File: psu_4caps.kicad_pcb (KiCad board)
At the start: 2 copper layers, 112.5 x 72.5 mm, 38 parts, among them J1 AC1, J10 GND, J11 V-, J12 V-, J2 GND2, J3 GND3, J4 AC4, J5 LED, J6 LED, J7 V+, J8 V+, J9 GND

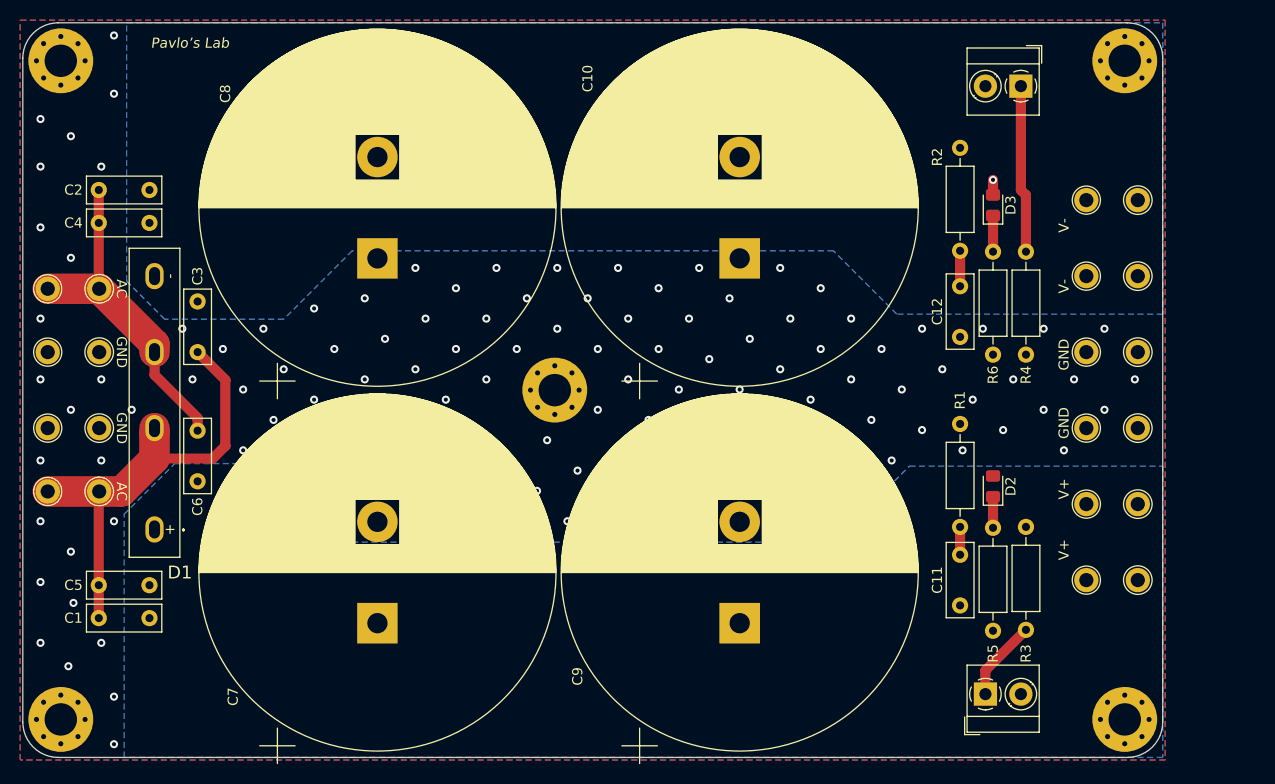
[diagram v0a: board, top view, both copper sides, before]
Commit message: rev2 commit
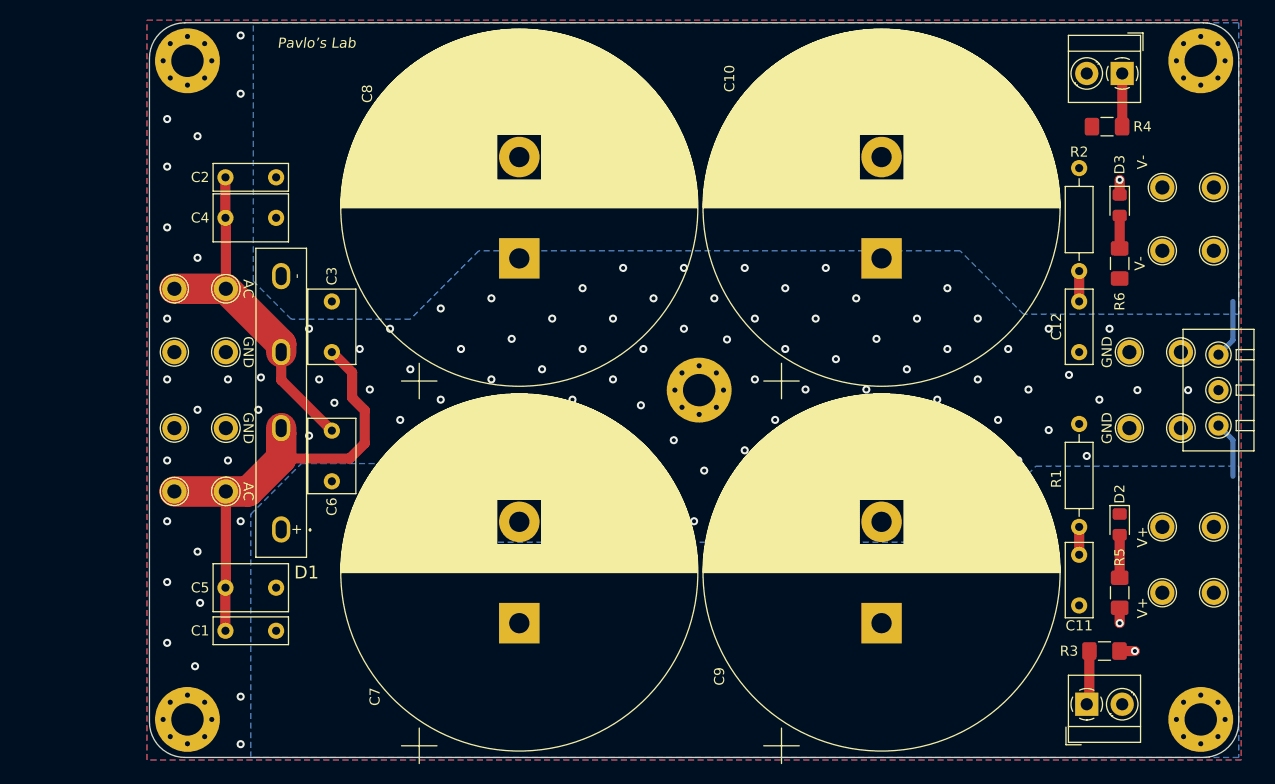
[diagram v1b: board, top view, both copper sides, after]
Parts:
- added J13: AUX OUT, local_footprints_lib:TerminalBlock_ Amphenol_01_03_P3.50mm, F.Cu at (143.0, 95.0)
- C3, C4, C5, C6: footprint Capacitor_THT:C_Rect_L7.2mm_W2.5mm_P5.00mm_FKS2_FKP2_MKS2_MKP2 -> Capacitor_THT:C_Rect_L7.2mm_W4.5mm_P5.00mm_FKS2_FKP2_MKS2_MKP2
- D2, D3: value LED -> LED_SMD; footprint Diode_SMD:D_0805_2012Metric_Pad1.15x1.40mm_HandSolder -> LED_SMD:LED_0805_2012Metric_Pad1.15x1.40mm_HandSolder
- R3, R4: footprint Resistor_THT:R_Axial_DIN0207_L6.3mm_D2.5mm_P10.16mm_Horizontal -> Resistor_SMD:R_1206_3216Metric_Pad1.42x1.75mm_HandSolder
- R5, R6: value 10K -> 47K; footprint Resistor_THT:R_Axial_DIN0207_L6.3mm_D2.5mm_P10.16mm_Horizontal -> Resistor_SMD:R_1206_3216Metric_Pad1.42x1.75mm_HandSolder
- moved R4 23.9 mm to (132.0, 69.0), turned to 0 degrees
- moved R6 15.4 mm to (133.2, 82.5)
- moved R3 14.5 mm to (131.8, 120.8), turned to 180 degrees
- moved H5 14.2 mm to (91.8, 95.0)
- moved C10 14.0 mm to (109.8, 82.0)
- moved C7 14.0 mm to (74.0, 118.0)
- moved C8 14.0 mm to (74.0, 82.0)
- moved C9 14.0 mm to (109.8, 118.0)
- moved C3 13.2 mm to (55.5, 91.2)
- moved C6 13.2 mm to (55.5, 104.0)
- moved D2 13.1 mm to (133.2, 108.2), turned to 270 degrees
- moved R5 13.1 mm to (133.2, 115.0)
- moved C1 12.6 mm to (45.0, 118.8)
- moved C2 12.6 mm to (45.0, 74.0)
- moved C4 12.5 mm to (50.0, 78.0)
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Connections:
- D2 pad 1: Net-(D2-Pad1) -> GND
- D2 pad 2: GND -> Net-(D2-Pad2)
- D3 pad 1: Net-(D3-Pad1) -> /V-
- D3 pad 2: /V- -> Net-(D3-Pad2)
- R5 pad 2: Net-(D2-Pad1) -> Net-(D2-Pad2)
- R6 pad 2: Net-(D3-Pad1) -> Net-(D3-Pad2)
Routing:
- net Net-(J6-Pad1): track 16.5 -> 5.24 mm
- net /V+: track 0.00 -> 8.62 mm, vias 0 -> 2
- net /V-: track 1.47 -> 7.32 mm
- net Net-(D2-Pad2): track 0.00 -> 4.24 mm
- net Net-(D3-Pad1): track 3.56 -> 0.00 mm
- net Net-(D3-Pad2): track 0.00 -> 3.24 mm
- net Net-(D2-Pad1): track 3.06 -> 0.00 mm
- net Net-(J5-Pad1): track 8.00 -> 5.36 mm
- net /AC1: track 45.3 -> 47.9 mm
- net /AC4: track 32.9 -> 34.5 mm
- net Net-(C12-Pad2): track 3.50 -> 3.00 mm
- net GND: vias 128 -> 117
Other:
- board size 112.5 x 72.5 mm -> 107.5 x 72.5 mm
- net class Default: clearance 0.2 -> 0.3; trace_width 0.25 -> 0.3; via_dia 0.8 -> 0.7; via_drill 0.4 -> 0.3
- rule trace_clearance: 0.2 -> 0.3
- rule trace_min: 0.2 -> 0.3
- rule via_min_size: 0.4 -> 0.3
- board text added: "Rev2.0"
- board text removed: "Rev1.0"

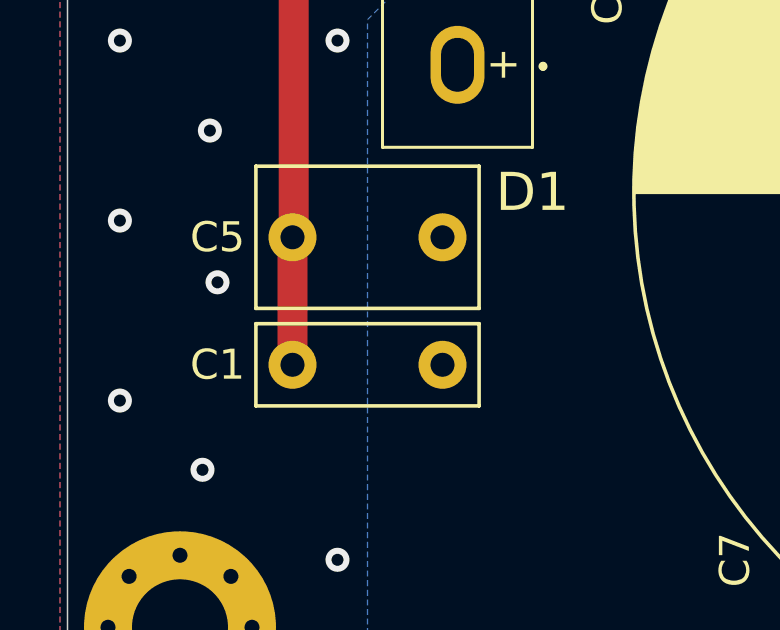
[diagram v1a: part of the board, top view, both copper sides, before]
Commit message: rev2 commit
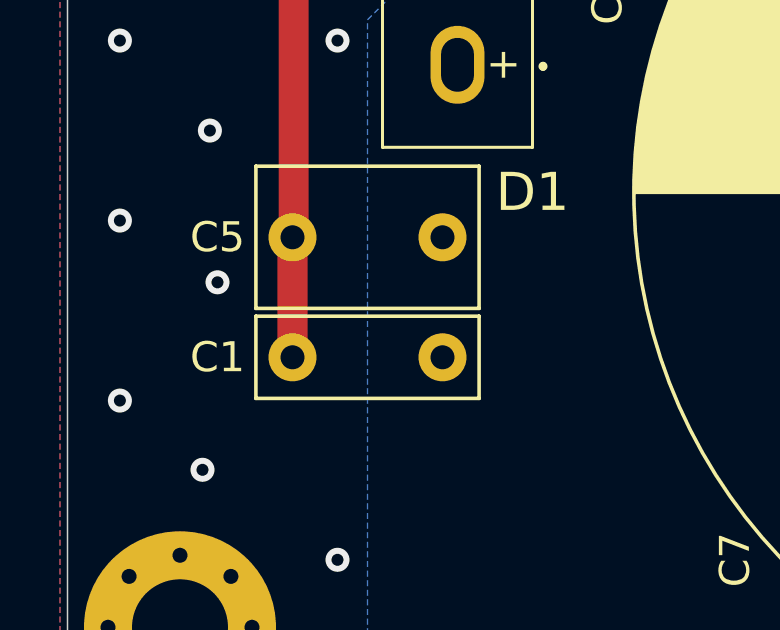
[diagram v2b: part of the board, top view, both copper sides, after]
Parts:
- moved C1 0.25 mm to (45.0, 118.5)
